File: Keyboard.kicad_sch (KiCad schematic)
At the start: 80 parts, among them J1 USB_C_Receptacle, J2 Conn_02x01_Row_Letter_First, K1 KEYSW, K10 KEYSW, K11 KEYSW, K12 KEYSW, K13 KEYSW, K14 KEYSW, K15 KEYSW, K16 KEYSW, K17 KEYSW, K18 KEYSW, K19 KEYSW, K2 KEYSW, K20 KEYSW, K21 KEYSW, K22 KEYSW, K23 KEYSW, K24 KEYSW, K25 KEYSW, K26 KEYSW, K27 KEYSW, K28 KEYSW, K29 KEYSW, K3 KEYSW, K30 KEYSW, K4 KEYSW, K5 KEYSW, K6 KEYSW, K7 KEYSW, K8 KEYSW, K9 KEYSW, U1 ESP32-C3FH4, U3 MCP73831-2-OT, U4 LM1117DT-3.3

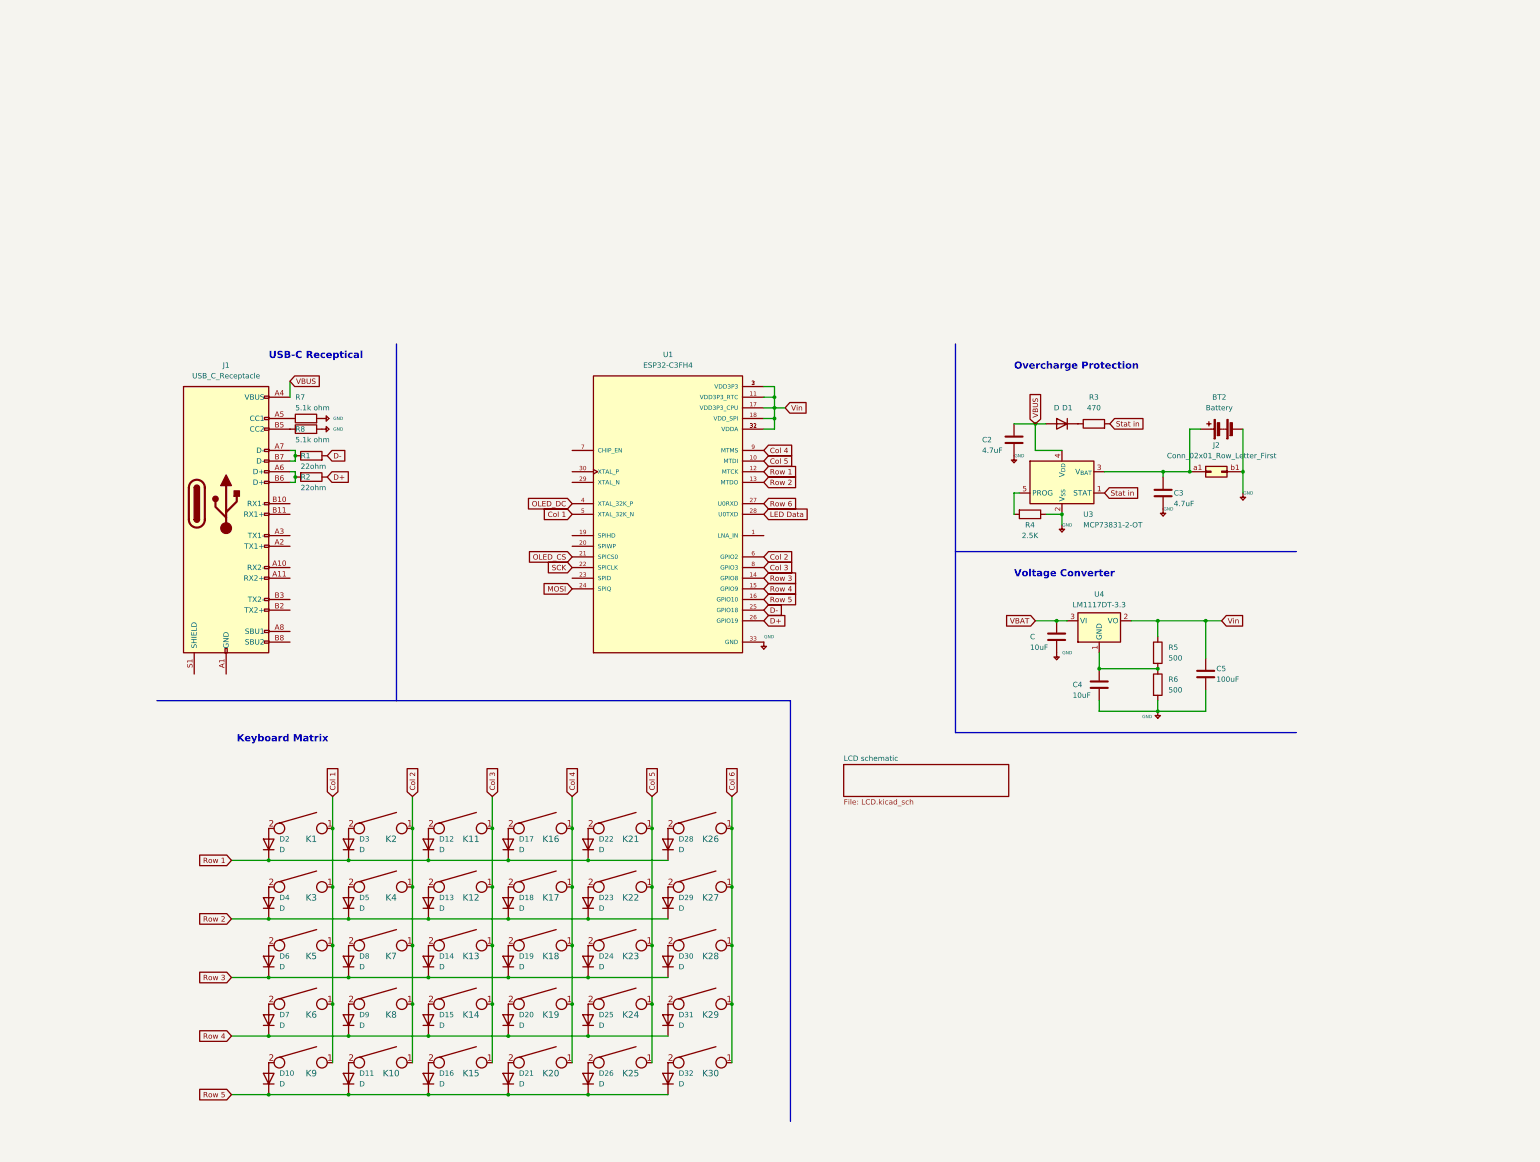
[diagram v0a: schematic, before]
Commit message: keyboard progress
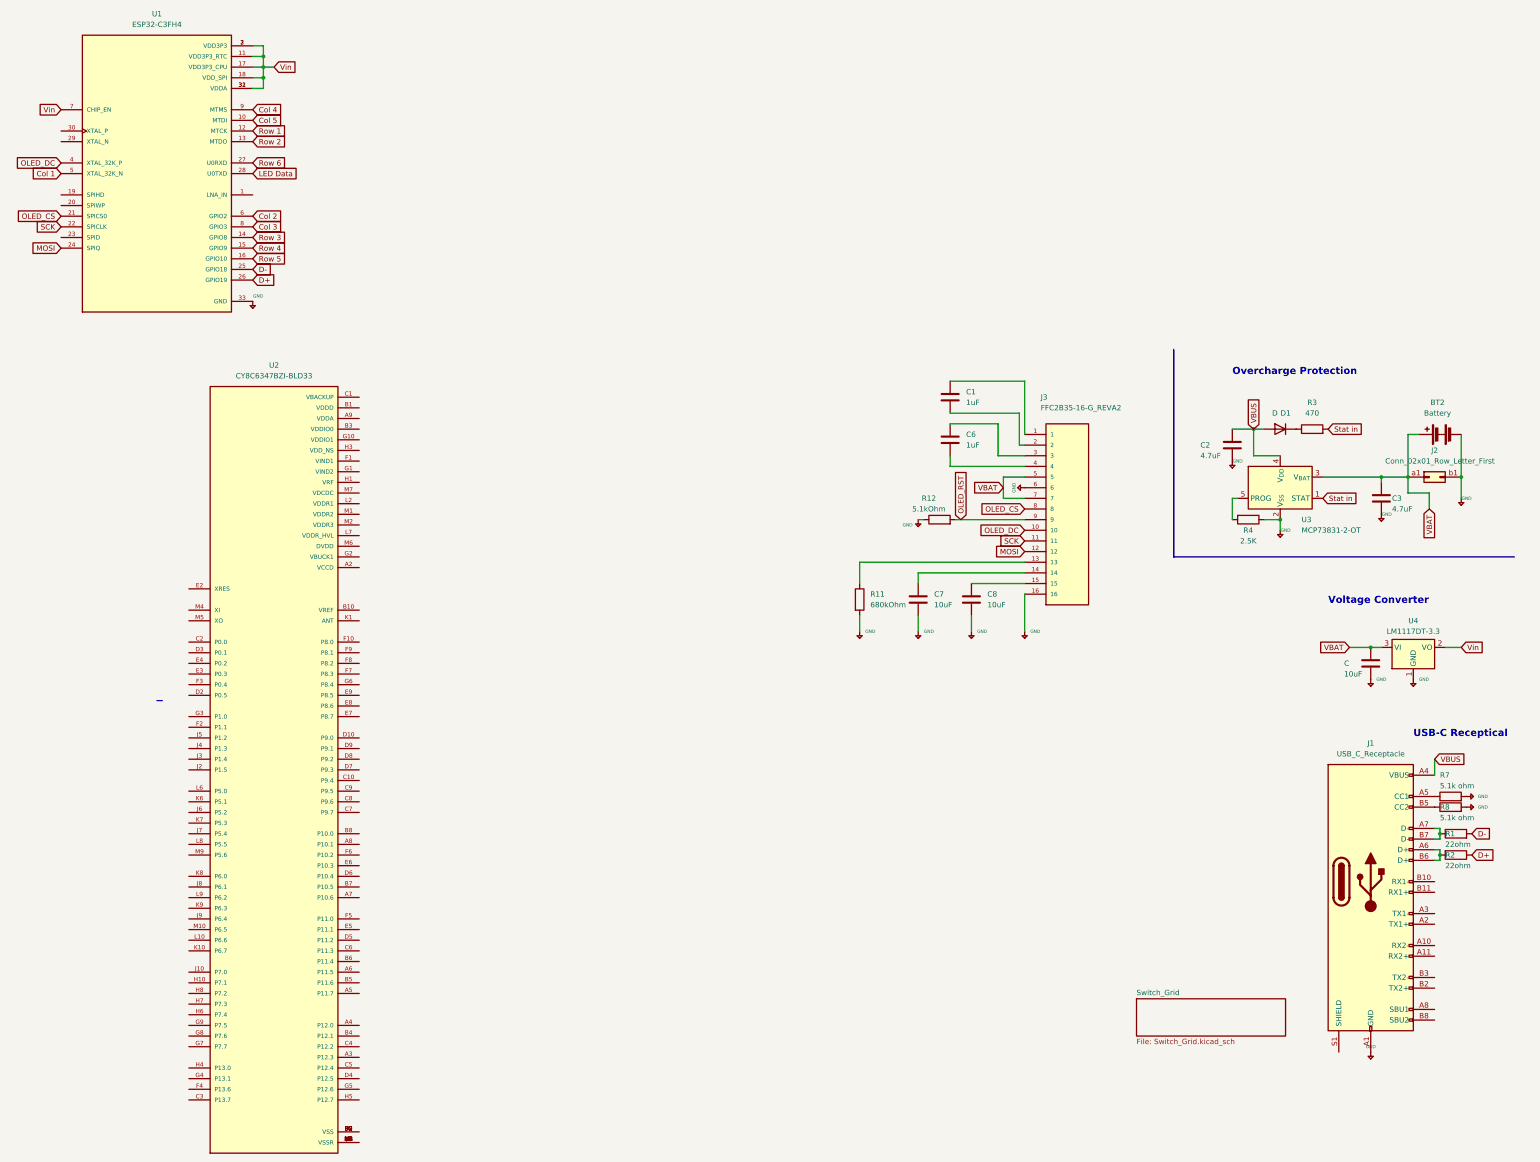
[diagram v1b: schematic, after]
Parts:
- removed C4: 10uF, symbol Device:C
- removed C5: 100uF, symbol Device:C
- removed D10, D11, D12, D13, D14, D15, D16, D17, D18, D19, D2, D20, D21, D22, D23, D24, D25, D26, D28, D29, D3, D30, D31, D32, D4, D5, D6, D7, D8, D9: D, symbol Device:D
- removed K1, K10, K11, K12, K13, K14, K15, K16, K17, K18, K19, K2, K20, K21, K22, K23, K24, K25, K26, K27, K28, K29, K3, K30, K4, K5, K6, K7, K8, K9: KEYSW, symbol keyboard_parts2:KEYSW
- removed R5, R6: 500, symbol Device:R
- added C1, C6: 1uF, symbol Device:C
- added C7, C8: 10uF, symbol Device:C
- added J3: FFC2B35-16-G_REVA2, FFC2B35-16-G_REVA2:GCT_FFC2B35-16-G_REVA2, symbol FFC2B35-16-G_REVA2:FFC2B35-16-G_REVA2
- added R11: 680kOhm, symbol Device:R
- added R12: 5.1kOhm, symbol Device:R
- added U2: CY8C6347BZI-BLD33, CY8C6347BZI-BLD33:BGA116N50P10X12_520X640X70N, symbol CY8C6347BZI-BLD33:CY8C6347BZI-BLD33
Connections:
- net +5V: now also J1.A1 (GND), J1.A12 (GND), J1.B1 (GND), J1.B12 (GND), U4.1 (GND), C7.2, C8.2, J3.16, J3.6, R11.2, R12.1
- net MOSI: now also J3.12
- net OLED_CS: now also J3.8
- net OLED_DC: now also J3.10
- net SCK: now also J3.11
- net VBAT: now also BT2.1 (+), C3.1, J2.a1 (Pin_a1), U3.3 (V_{BAT}), J3.5, J3.7
- net Vin: now also U1.7 (CHIP_EN)
- new net: C7.1, J3.14
- new net: C1.1, J3.1
- new net: J3.13, R11.1
- new net: C8.1, J3.15
- new net: C1.2, J3.2
- new net: C6.1, J3.3
- new net: C6.2, J3.4
- new net: U2.B2 (VSS), U2.B9 (VSS), U2.D1 (VSS), U2.H2 (VSS), U2.H9 (VSS)
- new net: U2.J1 (VSSR), U2.K2 (VSSR), U2.K3 (VSSR), U2.K4 (VSSR), U2.K5 (VSSR), U2.L1 (VSSR), U2.L3 (VSSR), U2.L4 (VSSR), U2.L5 (VSSR), U2.M3 (VSSR), U2.M8 (VSSR)
- new net OLED_RST: J3.9, R12.2
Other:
- removed sheet LCD schematic
- added sheet Switch_Grid (Switch_Grid.kicad_sch)
- note removed: "Keyboard Matrix"
- moved on the sheet: BT2, C, C2, C3, D1, J1, J2, R1, R2, R3, R4, R7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
